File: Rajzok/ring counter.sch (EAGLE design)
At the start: 17 parts, among them Q1 TP0602N2, Q2 TP0602N2, Q3 SUP75N06-08, Q4 SUP75N06-08

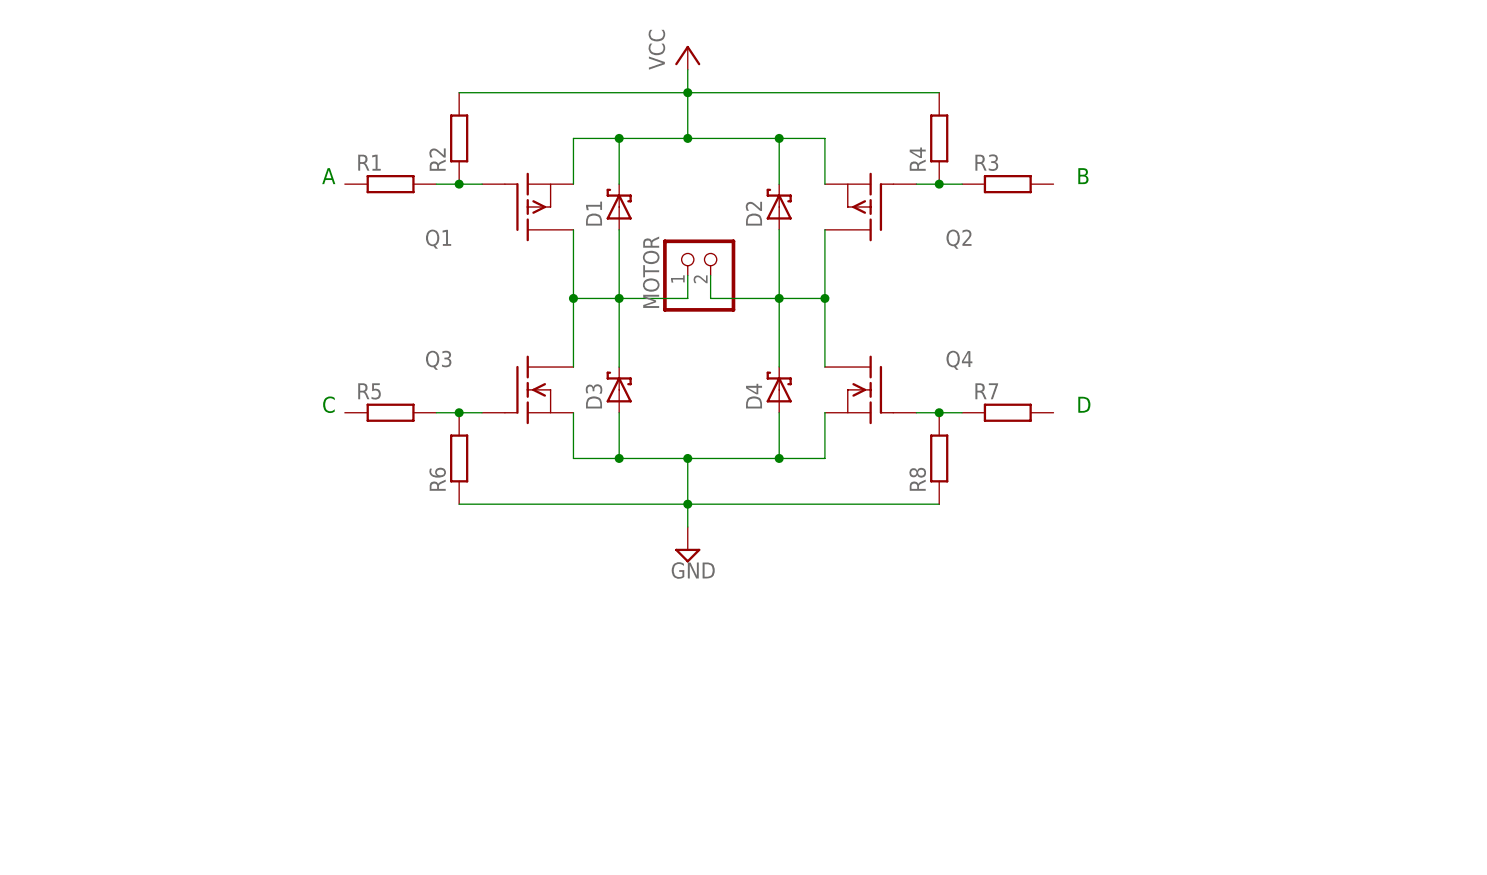
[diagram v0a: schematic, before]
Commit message: Rajzok 2017
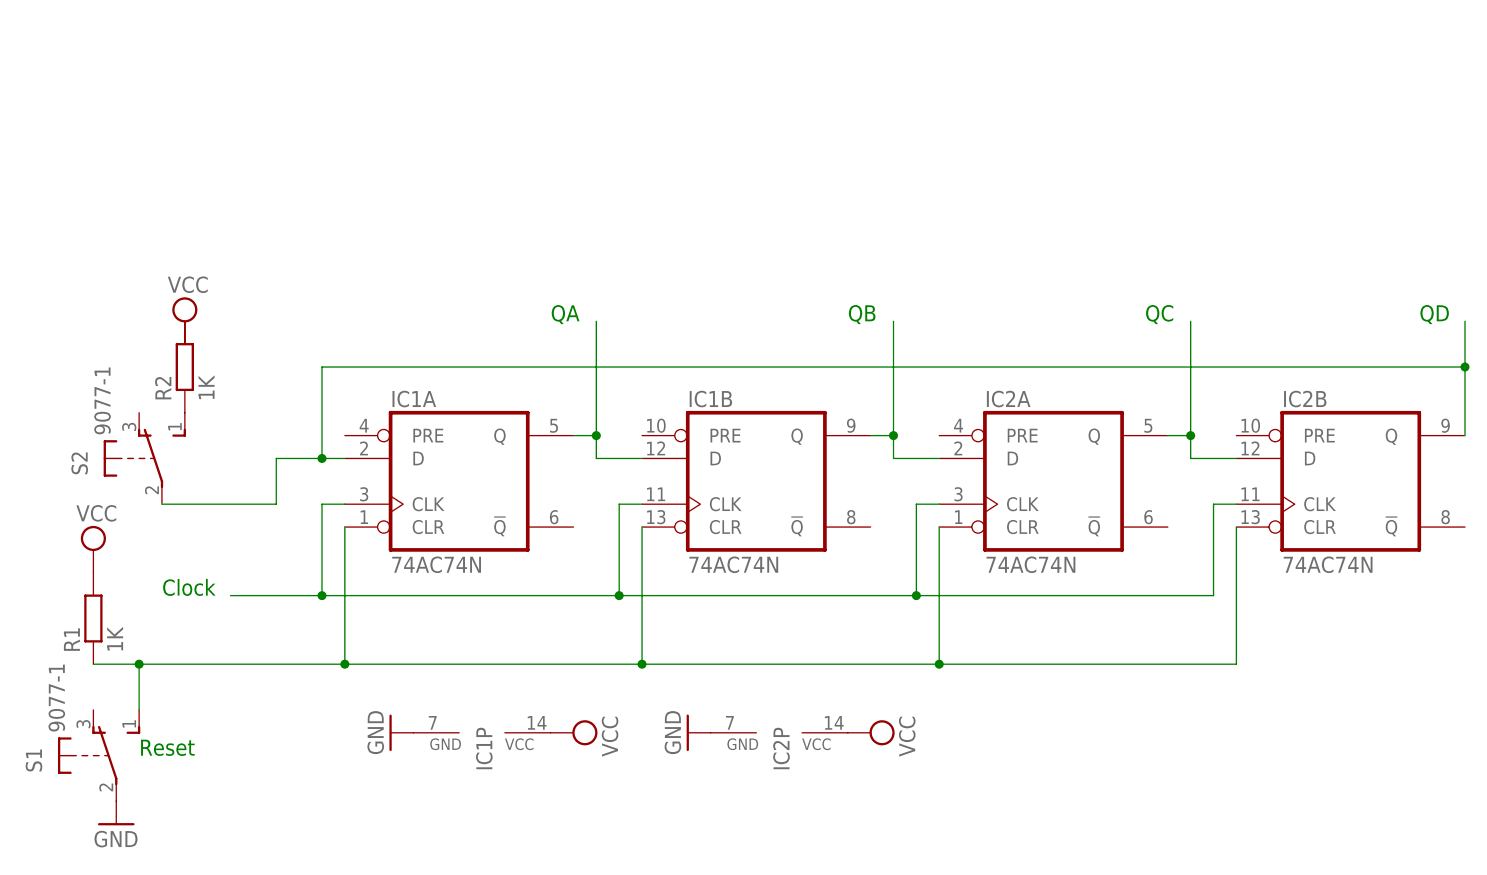
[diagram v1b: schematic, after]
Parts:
- removed D1, D2, D3, D4: 1N6267A, diode:1N6267A
- removed MOTOR: (no value), pinhead:PINHD-1X2
- removed Q1, Q2: TP0602N2, transistor-fet:TP0602N2
- removed Q3, Q4: SUP75N06-08, transistor-fet:SUP75N06-08
- removed R3, R4, R5, R6, R7, R8: (no value), rcl:R-EU_0204/7
- added IC1, IC2: 74AC74N, 74xx-eu:74AC74N
- added S1, S2: 9077-1, switch-misc:9077-1
- R1, R2: value (none) -> 1K
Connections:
- removed net N$9: D1.A, D3.C, MOTOR.1, Q1.D, Q3.D
- new net CLOCK: IC1A.CLK, IC1B.CLK, IC2A.CLK, IC2B.CLK
- new net N$6: IC1A.CLR, IC1B.CLR, IC2A.CLR, IC2B.CLR, R1.1, S1.S
- net GND: now also IC1P.GND, IC2P.GND, S1.P; no longer D3.A, D4.A, Q3.S, Q4.S, R6.1, R8.1
- net N$1: now also IC1A.Q, IC1B.D; no longer Q1.G, R1.2, R2.1
- net N$2: now also IC1B.Q, IC2A.D; no longer D2.A, D4.C, MOTOR.2, Q2.D, Q4.D
- net N$3: now also IC2A.Q, IC2B.D; no longer Q2.G, R3.1, R4.1
- net N$4: now also R2.1, S2.S; no longer Q3.G, R5.2, R6.2
- net N$5: now also IC1A.D, IC2B.Q, S2.P; no longer Q4.G, R7.1, R8.2
- net VCC: now also IC1P.VCC, IC2P.VCC, R1.2; no longer D1.C, D2.C, Q1.S, Q2.S, R2.2, R4.2
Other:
- note added: "Clock"
- note added: "QA"
- note added: "QB"
- note added: "QC"
- note added: "QD"
- note added: "Reset"
- note removed: "A"
- note removed: "B"
- note removed: "C"
- note removed: "D"
- moved on the sheet: R1, R2
